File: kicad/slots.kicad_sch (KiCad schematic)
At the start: 98 parts, among them J19 2.54-2*3P, J20 2.54-2*3P, J3 WingTAT 2044-2X32G00SA, J5 WingTAT 2044-2X32G00SA, J53 XFCN PM254V-11-07-H85, J54 XFCN PM254V-11-07-H85, J55 XFCN PM254V-11-07-H85, J56 XFCN PM254V-11-07-H85, J57 XFCN PM254V-11-07-H85, J58 XFCN PM254V-11-07-H85, J62 XFCN PM254V-11-07-H85, J63 XFCN PM254V-11-07-H85, J64 XFCN PM254V-11-07-H85, J65 XFCN PM254V-11-07-H85, J7 PM254-2-08-Z-8.5, J8 PM254-2-08-Z-8.5, U10 SN74LXC8T245PWR, U9 SN74LXC8T245PWR

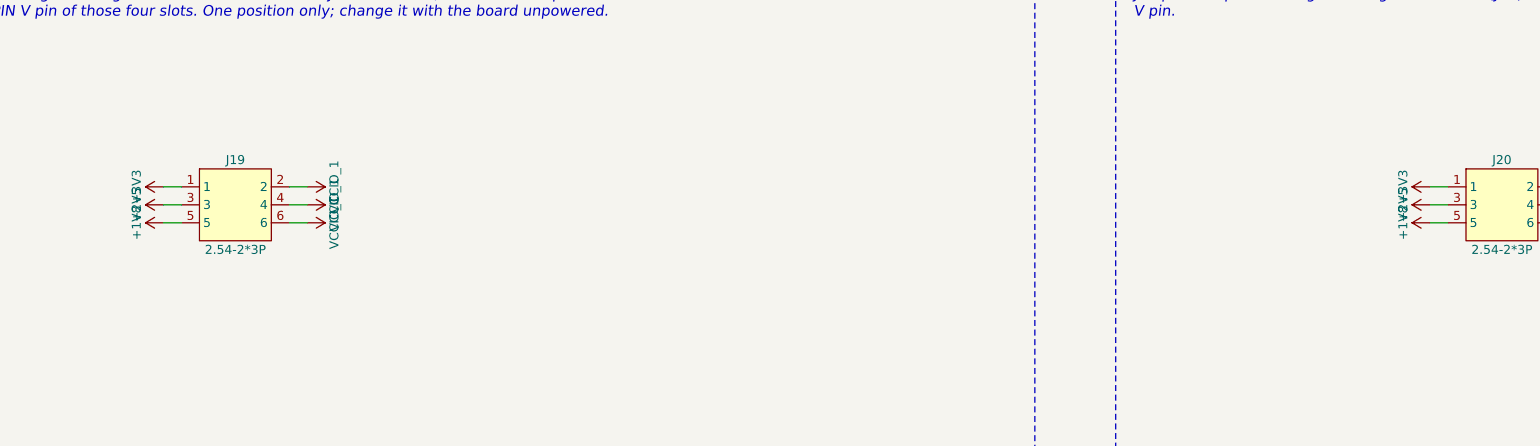
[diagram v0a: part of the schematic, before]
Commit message: Step 1: the +1V8_IO rail
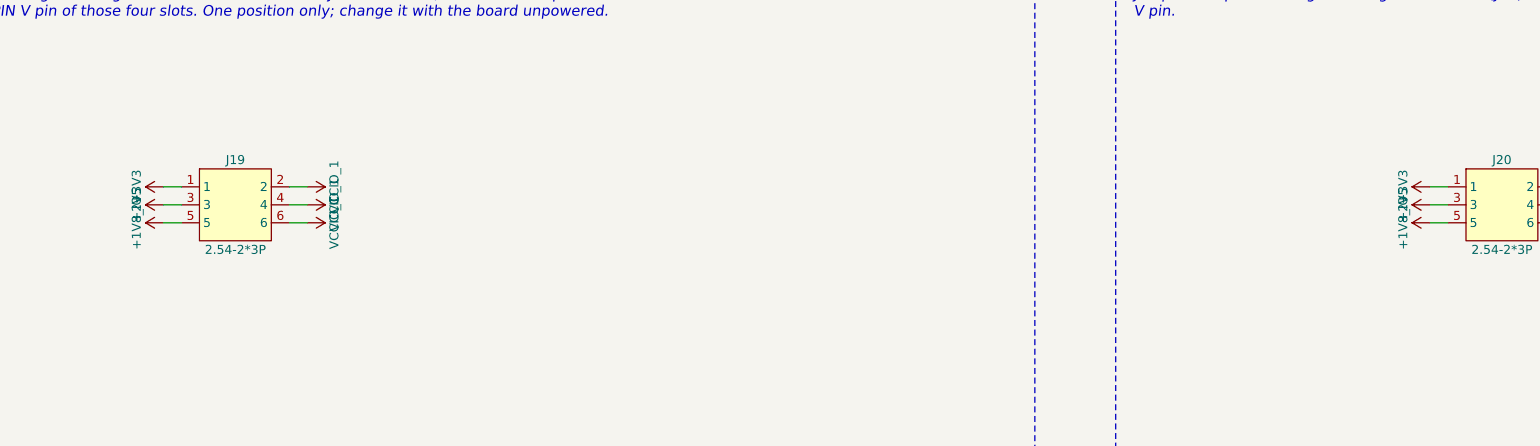
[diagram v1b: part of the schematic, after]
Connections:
- net +1V8 renamed +1V8_IO
